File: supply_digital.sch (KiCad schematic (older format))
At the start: 20 parts

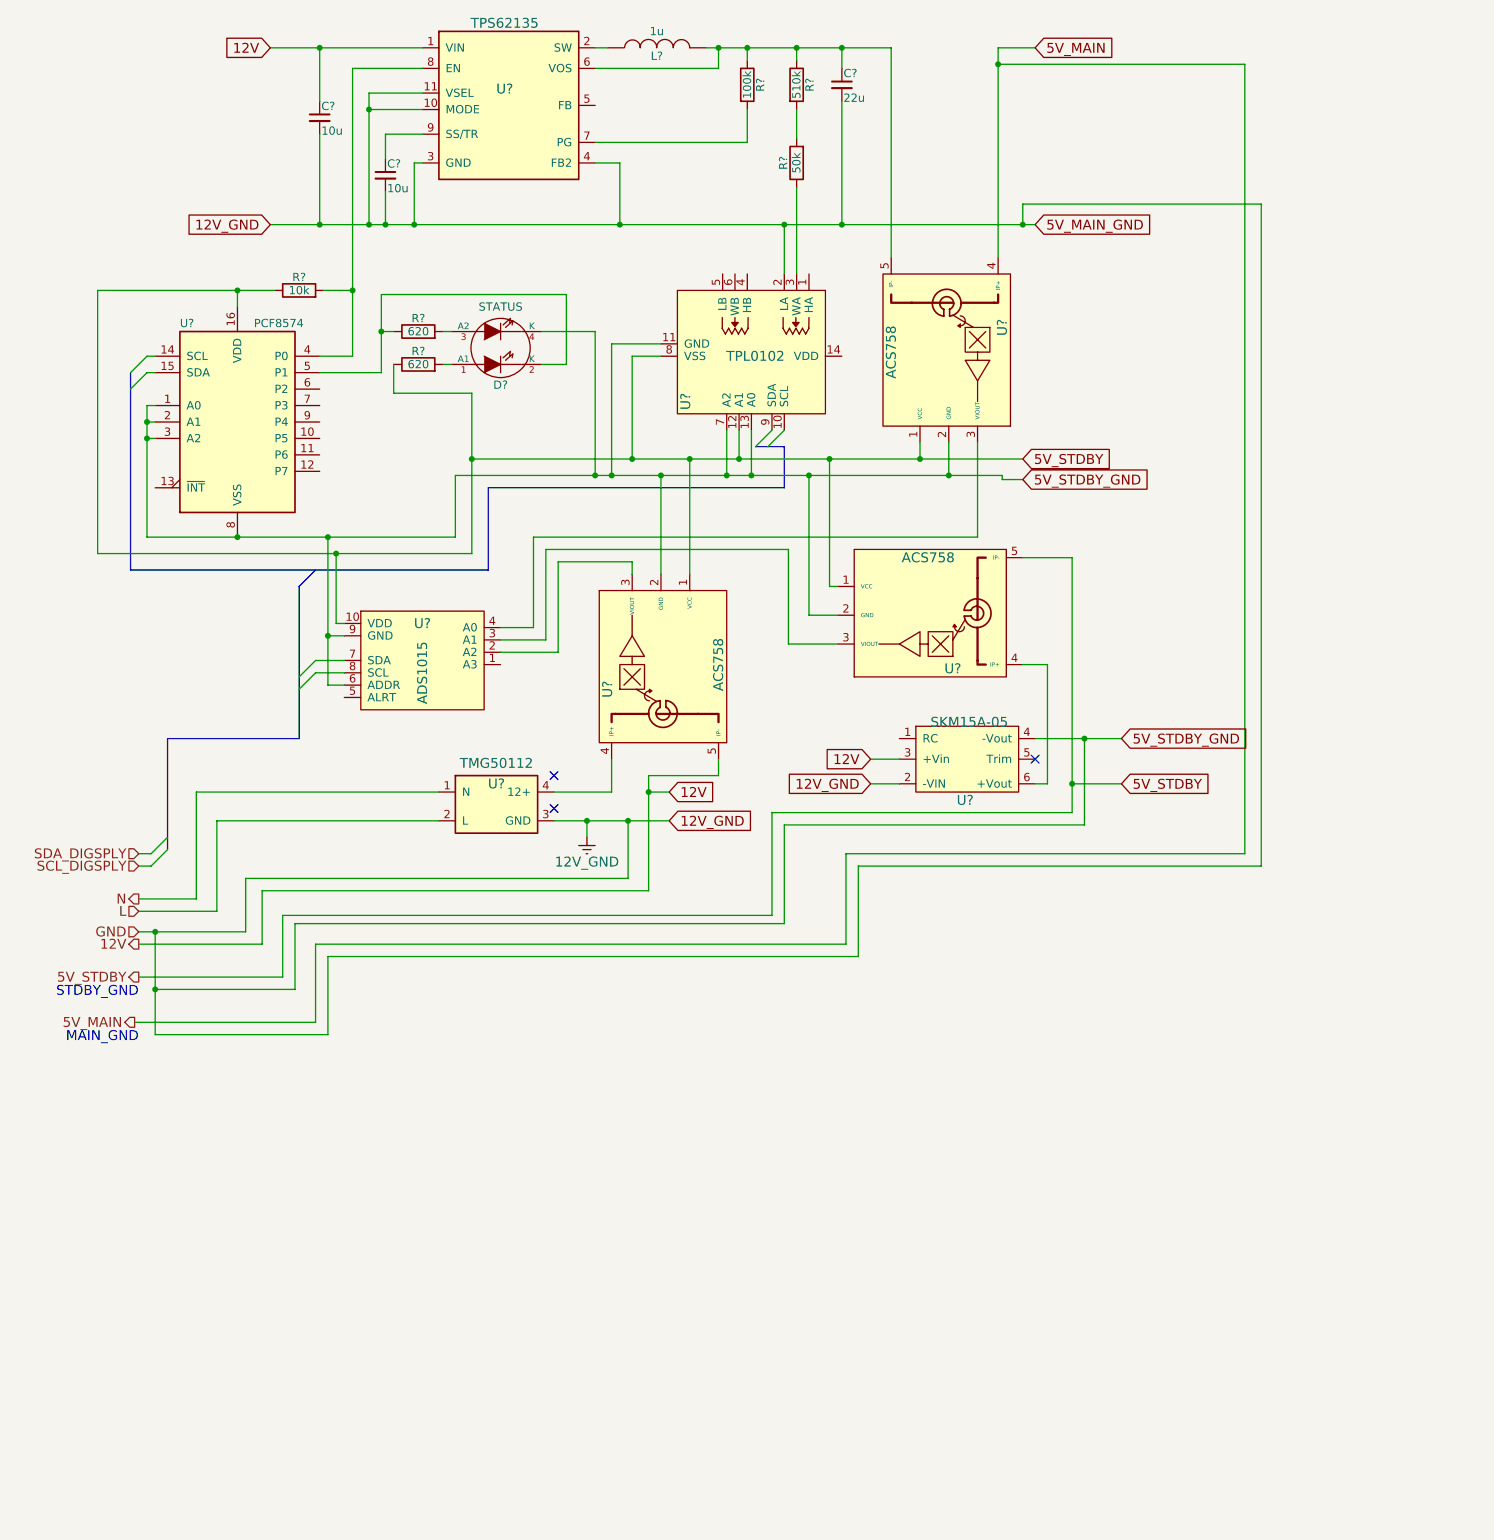
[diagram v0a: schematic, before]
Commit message: blub
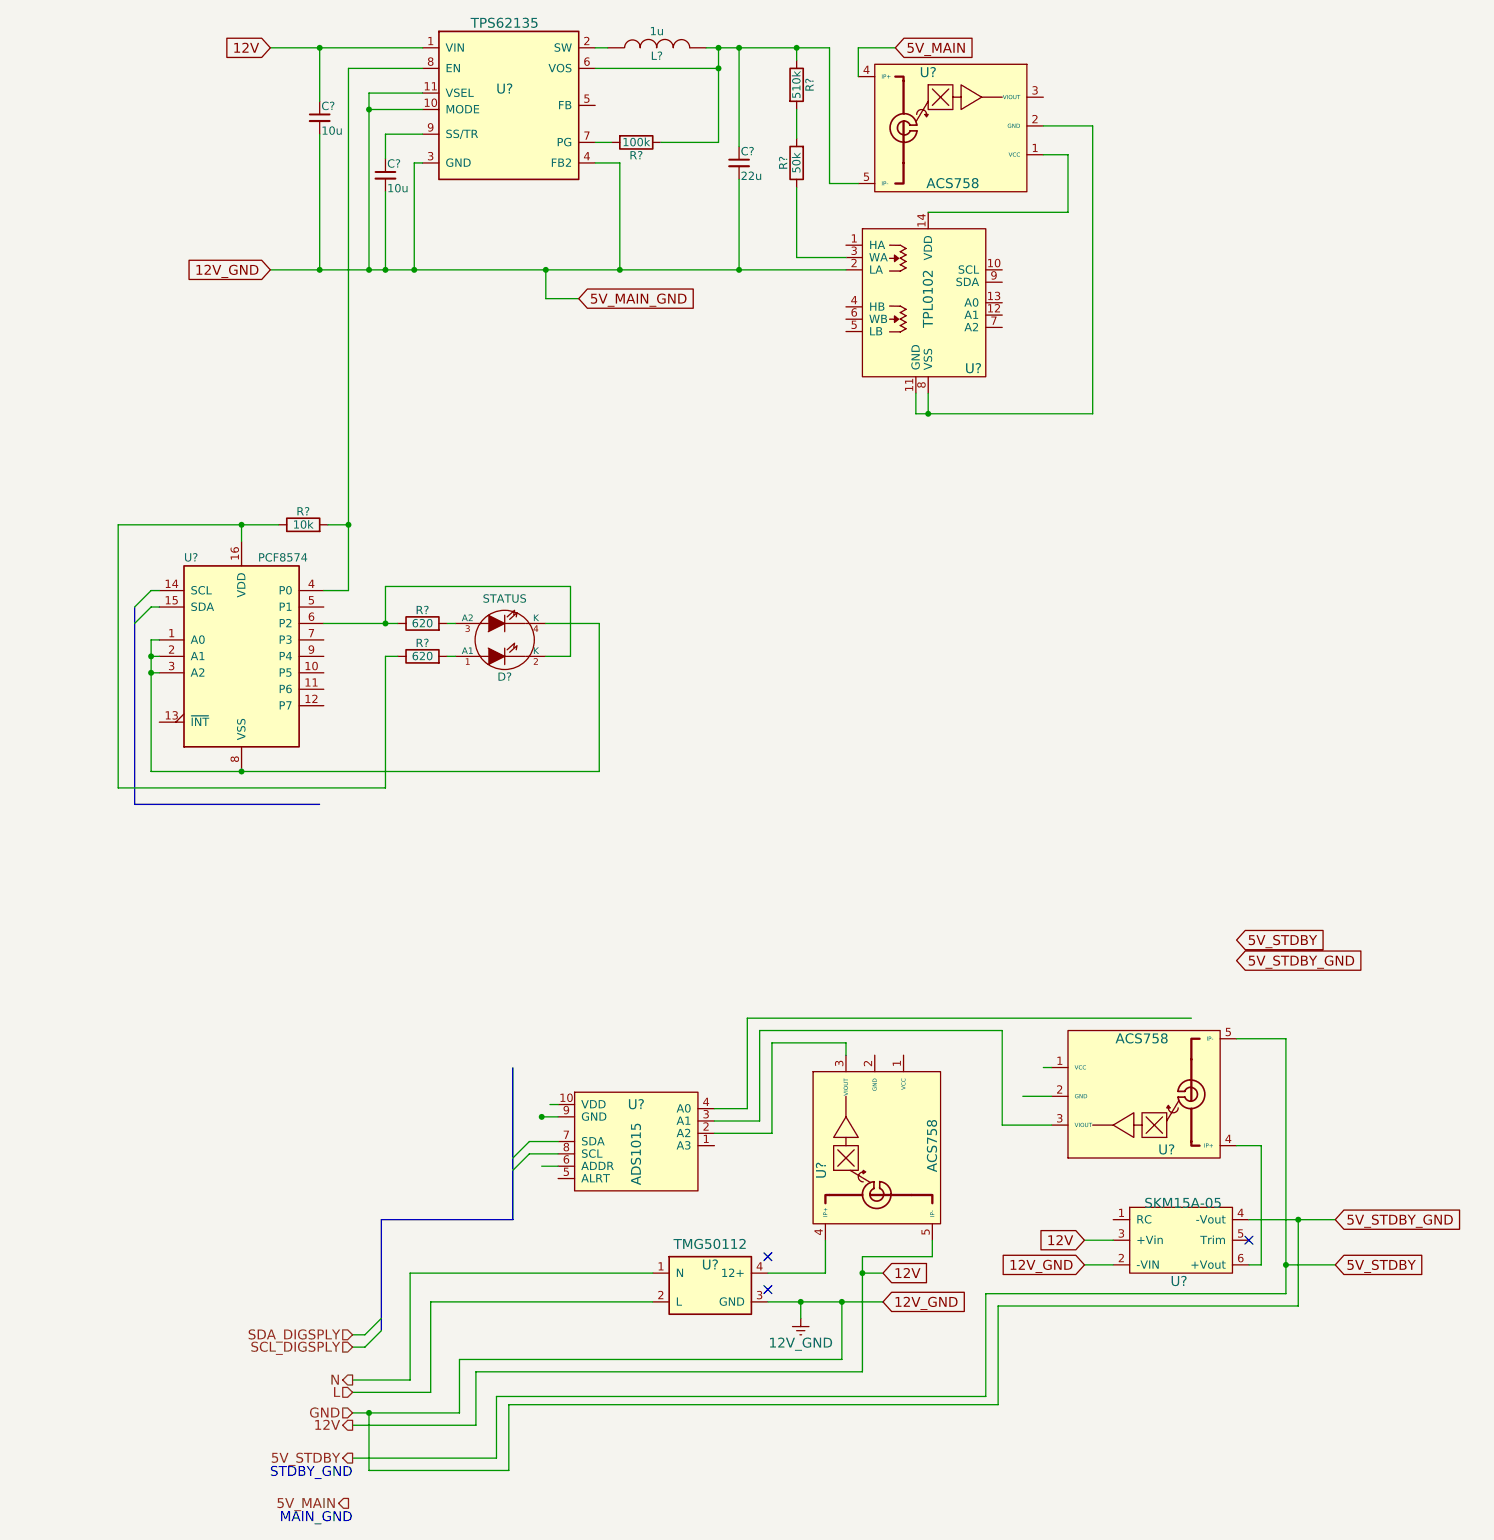
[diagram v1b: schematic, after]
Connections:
- wire segments 157 -> 129
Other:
- moved on the sheet: C?, D?, R?, U?

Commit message: daily commit
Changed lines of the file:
@@
 	7175 1575 7475 1575
 Wire Wire Line
-	7475 3325 7475 1575
+	7475 1575 7475 3325
 Wire Wire Line
-	6400 3325 7475 3325
+	7475 3325 6400 3325
 Wire Wire Line
 	6400 3325 6400 3200
